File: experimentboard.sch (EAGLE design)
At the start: 173 parts, among them IC1 TL072P, IC2 LM317, IC3 LM337, IC4 TL072P, IC5 TL072P, IC6 TL072P, P1 PLR135/T9, U1 PCM1690, U2 DIR9001, U3 CAT24C256

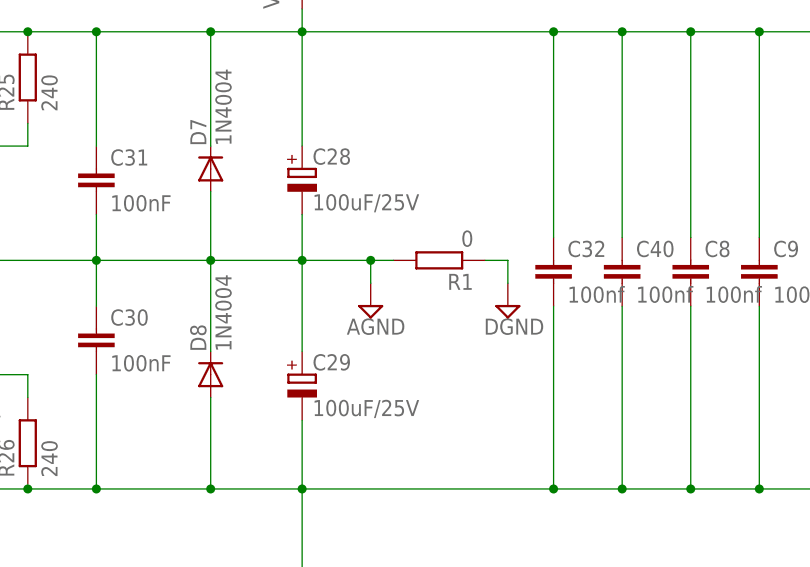
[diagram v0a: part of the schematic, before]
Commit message: Very nearly done
I added some power and ground planes and finished more routing.

Still a bit of decision making to do before I can finish it.
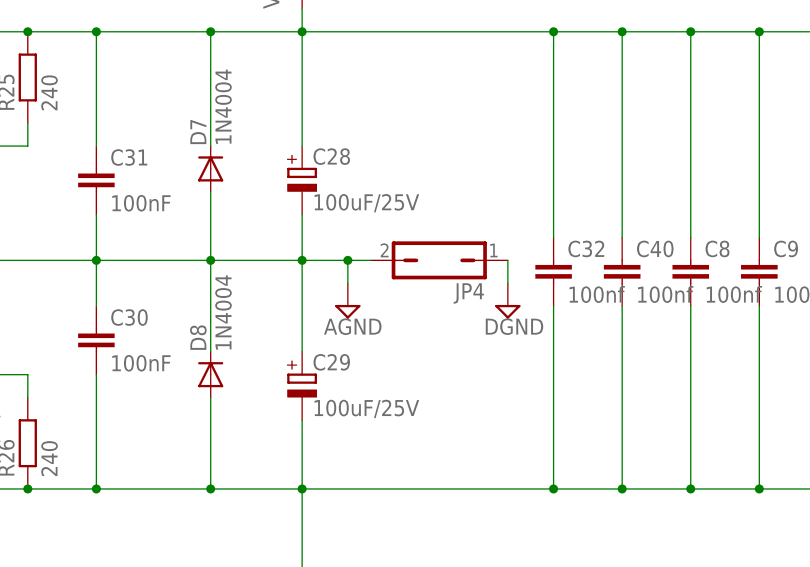
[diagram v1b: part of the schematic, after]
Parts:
- removed R1: 0, rcl:R-EU_0207/10
- added JP4: (no value), jumper:JP1Q
- P9: value BEAGLEBONEP9 -> P9
- renumbered U$2 to P9
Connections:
- net AGND: now also JP4.2; no longer R1.2
- net DGND: now also JP4.1; no longer R1.1
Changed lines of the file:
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@@
 <part name="R32" library="rcl" deviceset="R-EU_" device="0207/7" value="22"/>
 <part name="R3" library="rcl" deviceset="R-EU_" device="0207/7" value="10k"/>
-<part name="U$2" library="0000halfgaar" deviceset="BEAGLEBONEP9" device=""/>
+<part name="P9" library="0000halfgaar" deviceset="BEAGLEBONEP9" device="" value="P9"/>
 <part name="R35" library="rcl" deviceset="R-EU_" device="0207/7" value="22"/>
 <part name="R36" library="rcl" deviceset="R-EU_" device="0207/7" value="22"/>
@@
 <part name="SUPPLY14" library="supply2" deviceset="VDD" device=""/>
 <part name="SUPPLY31" library="supply2" deviceset="VDD" device=""/>
-<part name="R1" library="rcl" deviceset="R-EU_" device="0207/10" value="0"/>
 <part name="SUPPLY13" library="supply2" deviceset="DGND" device=""/>
 <part name="SUPPLY27" library="supply2" deviceset="VCC" device=""/>
@@
 <part name="C16" library="rcl" deviceset="CPOL-EU" device="E2-5" value="10 µF"/>
 <part name="C17" library="rcl" deviceset="CPOL-EU" device="E2-5" value="10 µF"/>
+<part name="JP4" library="jumper" deviceset="JP1Q" device=""/>
 </parts>
 <sheets>
@@
 </instance>
 <instance part="SUPPLY15" gate="G$1" x="-81.28" y="93.98" rot="R180"/>
-<instance part="SUPPLY16" gate="G$1" x="116.84" y="210.82"/>
+<instance part="SUPPLY16" gate="G$1" x="114.3" y="210.82"/>
 <instance part="AOUT" gate="-1" x="309.88" y="152.4" rot="R180"/>
 <instance part="AOUT" gate="-2" x="309.88" y="162.56" rot="R180"/>
@@
 <attribute name="VALUE" x="62.23" y="4.318" size="1.778" layer="96"/>
 </instance>
-<instance part="U$2" gate="G$1" x="-50.8" y="58.42"/>
+<instance part="P9" gate="G$1" x="-50.8" y="58.42"/>
 <instance part="R35" gate="G$1" x="63.5" y="93.98" smashed="yes">
 <attribute name="NAME" x="67.056" y="91.6686" size="1.778" layer="95"/>
@@
 <instance part="SUPPLY14" gate="G$1" x="22.86" y="43.18"/>
 <instance part="SUPPLY31" gate="G$1" x="30.48" y="43.18"/>
-<instance part="R1" gate="G$1" x="124.46" y="215.9" rot="R180"/>
 <instance part="SUPPLY13" gate="G$1" x="132.08" y="210.82"/>
 <instance part="SUPPLY27" gate="G$1" x="210.82" y="238.76" rot="R180"/>
@@
 <instance part="C16" gate="G$1" x="96.52" y="-187.96" rot="R90"/>
 <instance part="C17" gate="G$1" x="165.1" y="-83.82"/>
+<instance part="JP4" gate="A" x="124.46" y="215.9" rot="R90"/>
 </instances>
 <busses>
@@
 <pinref part="R32" gate="G$1" pin="1"/>
 <wire x1="68.58" y1="-119.38" x2="-15.24" y2="-119.38" width="0.1524" layer="91"/>
-<pinref part="U$2" gate="G$1" pin="DIN"/>
+<pinref part="P9" gate="G$1" pin="DIN"/>
 <wire x1="-30.48" y1="68.58" x2="-15.24" y2="68.58" width="0.1524" layer="91"/>
 <wire x1="-15.24" y1="68.58" x2="-15.24" y2="-119.38" width="0.1524" layer="91"/>
@@
 </segment>
 <segment>
-<pinref part="U$2" gate="G$1" pin="3.3V"/>
+<pinref part="P9" gate="G$1" pin="3.3V"/>
 <pinref part="SUPPLY19" gate="G$1" pin="VDD"/>
 <wire x1="-78.74" y1="86.36" x2="-91.44" y2="86.36" width="0.1524" layer="91"/>
@@
 </segment>
 <segment>
-<pinref part="U$2" gate="G$1" pin="DGND"/>
+<pinref part="P9" gate="G$1" pin="DGND"/>
 <pinref part="SUPPLY15" gate="G$1" pin="DGND"/>
 <wire x1="-78.74" y1="88.9" x2="-81.28" y2="88.9" width="0.1524" layer="91"/>
@@
 </segment>
 <segment>
-<pinref part="R1" gate="G$1" pin="1"/>
 <pinref part="SUPPLY13" gate="G$1" pin="DGND"/>
-<wire x1="129.54" y1="215.9" x2="132.08" y2="215.9" width="0.1524" layer="91"/>
 <wire x1="132.08" y1="215.9" x2="132.08" y2="213.36" width="0.1524" layer="91"/>
+<pinref part="JP4" gate="A" pin="1"/>
 </segment>
 <segment>
@@
 </segment>
 <segment>
-<wire x1="116.84" y1="215.9" x2="116.84" y2="213.36" width="0.1524" layer="91"/>
+<wire x1="114.3" y1="215.9" x2="114.3" y2="213.36" width="0.1524" layer="91"/>
 <wire x1="109.22" y1="205.74" x2="109.22" y2="215.9" width="0.1524" layer="91"/>
 <wire x1="109.22" y1="215.9" x2="109.22" y2="220.98" width="0.1524" layer="91"/>
-<wire x1="109.22" y1="215.9" x2="116.84" y2="215.9" width="0.1524" layer="91"/>
+<wire x1="109.22" y1="215.9" x2="114.3" y2="215.9" width="0.1524" layer="91"/>
 <wire x1="99.06" y1="205.74" x2="99.06" y2="215.9" width="0.1524" layer="91"/>
 <wire x1="99.06" y1="215.9" x2="99.06" y2="223.52" width="0.1524" layer="91"/>
@@
 <wire x1="55.88" y1="223.52" x2="55.88" y2="215.9" width="0.1524" layer="91"/>
 <pinref part="SUPPLY16" gate="G$1" pin="AGND"/>
-<pinref part="R1" gate="G$1" pin="2"/>
-<wire x1="119.38" y1="215.9" x2="116.84" y2="215.9" width="0.1524" layer="91"/>
-<junction x="116.84" y="215.9"/>
+<pinref part="JP4" gate="A" pin="2"/>
+<wire x1="116.84" y1="215.9" x2="114.3" y2="215.9" width="0.1524" layer="91"/>
+<junction x="114.3" y="215.9"/>
 </segment>
 <segment>
@@
 <wire x1="22.86" y1="17.78" x2="10.16" y2="17.78" width="0.1524" layer="91"/>
 <wire x1="10.16" y1="17.78" x2="10.16" y2="58.42" width="0.1524" layer="91"/>
-<pinref part="U$2" gate="G$1" pin="I2C_SCL"/>
+<pinref part="P9" gate="G$1" pin="I2C_SCL"/>
 <wire x1="10.16" y1="58.42" x2="-30.48" y2="58.42" width="0.1524" layer="91"/>
 <pinref part="R38" gate="G$1" pin="1"/>
@@
 <wire x1="30.48" y1="22.86" x2="76.2" y2="22.86" width="0.1524" layer="91"/>
 <wire x1="12.7" y1="22.86" x2="12.7" y2="55.88" width="0.1524" layer="91"/>
-<pinref part="U$2" gate="G$1" pin="I2C_SDA"/>
+<pinref part="P9" gate="G$1" pin="I2C_SDA"/>
 <wire x1="12.7" y1="55.88" x2="-30.48" y2="55.88" width="0.1524" layer="91"/>
 <pinref part="R39" gate="G$1" pin="1"/>
@@
 </segment>
 <segment>
-<pinref part="U$2" gate="G$1" pin="VDD_5V"/>
+<pinref part="P9" gate="G$1" pin="VDD_5V"/>
 <pinref part="SUPPLY28" gate="G$1" pin="VCC"/>
 <wire x1="-78.74" y1="83.82" x2="-101.6" y2="83.82" width="0.1524" layer="91"/>
@@
 <wire x1="17.78" y1="66.04" x2="-7.62" y2="66.04" width="0.1524" layer="91"/>
 <wire x1="-7.62" y1="66.04" x2="-7.62" y2="86.36" width="0.1524" layer="91"/>
-<pinref part="U$2" gate="G$1" pin="AHCLKX"/>
+<pinref part="P9" gate="G$1" pin="AHCLKX"/>
 <wire x1="-7.62" y1="86.36" x2="-30.48" y2="86.36" width="0.1524" layer="91"/>
 </segment>
@@
 <wire x1="68.58" y1="-109.22" x2="-12.7" y2="-109.22" width="0.1524" layer="91"/>
 <wire x1="-12.7" y1="-109.22" x2="-12.7" y2="71.12" width="0.1524" layer="91"/>
-<pinref part="U$2" gate="G$1" pin="FSR"/>
+<pinref part="P9" gate="G$1" pin="FSR"/>
 <wire x1="-12.7" y1="71.12" x2="-30.48" y2="71.12" width="0.1524" layer="91"/>
 </segment>
@@
 <segment>
 <pinref part="U1" gate="U$1" pin="RST"/>
-<pinref part="U$2" gate="G$1" pin="RESET(GPIO1_16)"/>
+<pinref part="P9" gate="G$1" pin="RESET(GPIO1_16)"/>
 <wire x1="-30.48" y1="50.8" x2="-2.54" y2="50.8" width="0.1524" layer="91"/>
 <wire x1="-2.54" y1="50.8" x2="-2.54" y2="48.26" width="0.1524" layer="91"/>
@@
 <pinref part="R31" gate="G$1" pin="1"/>
 <wire x1="68.58" y1="-114.3" x2="-10.16" y2="-114.3" width="0.1524" layer="91"/>
-<pinref part="U$2" gate="G$1" pin="ACLKR"/>
+<pinref part="P9" gate="G$1" pin="ACLKR"/>
 <wire x1="-30.48" y1="73.66" x2="-10.16" y2="73.66" width="0.1524" layer="91"/>
 <wire x1="-10.16" y1="73.66" x2="-10.16" y2="-114.3" width="0.1524" layer="91"/>
@@
 <net name="DOUT" class="0">
 <segment>
-<pinref part="U$2" gate="G$1" pin="DOUT"/>
+<pinref part="P9" gate="G$1" pin="DOUT"/>
 <wire x1="-30.48" y1="78.74" x2="7.62" y2="78.74" width="0.1524" layer="91"/>
 <wire x1="7.62" y1="78.74" x2="7.62" y2="83.82" width="0.1524" layer="91"/>
@@
 <net name="AHCLKX" class="0">
 <segment>
-<pinref part="U$2" gate="G$1" pin="FSX"/>
+<pinref part="P9" gate="G$1" pin="FSX"/>
 <wire x1="-30.48" y1="81.28" x2="-2.54" y2="81.28" width="0.1524" layer="91"/>
 <wire x1="-2.54" y1="81.28" x2="-2.54" y2="93.98" width="0.1524" layer="91"/>
@@
 <segment>
 <wire x1="2.54" y1="88.9" x2="2.54" y2="83.82" width="0.1524" layer="91"/>
-<pinref part="U$2" gate="G$1" pin="ACLKX"/>
+<pinref part="P9" gate="G$1" pin="ACLKX"/>
 <wire x1="2.54" y1="83.82" x2="-30.48" y2="83.82" width="0.1524" layer="91"/>
 <pinref part="R36" gate="G$1" pin="1"/>
@@
 <wire x1="83.82" y1="-63.5" x2="-17.78" y2="-63.5" width="0.1524" layer="91"/>
 <wire x1="-17.78" y1="-63.5" x2="-17.78" y2="66.04" width="0.1524" layer="91"/>
-<pinref part="U$2" gate="G$1" pin="DIR_AUDIO(GPIO1_19)"/>
+<pinref part="P9" gate="G$1" pin="DIR_AUDIO(GPIO1_19)"/>
 <wire x1="-17.78" y1="66.04" x2="-30.48" y2="66.04" width="0.1524" layer="91"/>
 </segment>
@@
 <net name="CAPE_I2C_SDA" class="0">
 <segment>
-<pinref part="U$2" gate="G$1" pin="EEPROM_I2C_SDA"/>
+<pinref part="P9" gate="G$1" pin="EEPROM_I2C_SDA"/>
 <wire x1="-30.48" y1="40.64" x2="-27.94" y2="40.64" width="0.1524" layer="91"/>
 <wire x1="-27.94" y1="40.64" x2="-27.94" y2="0" width="0.1524" layer="91"/>
@@
 <wire x1="-38.1" y1="2.54" x2="-25.4" y2="2.54" width="0.1524" layer="91"/>
 <wire x1="-25.4" y1="2.54" x2="-25.4" y2="43.18" width="0.1524" layer="91"/>
-<pinref part="U$2" gate="G$1" pin="EEPROM_I2C_SCL"/>
+<pinref part="P9" gate="G$1" pin="EEPROM_I2C_SCL"/>
 <wire x1="-25.4" y1="43.18" x2="-30.48" y2="43.18" width="0.1524" layer="91"/>
 <pinref part="R8" gate="G$1" pin="1"/>

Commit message: Fixed 5mm caps, fixed DRC errors
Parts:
- 1_C1, 1_C2, 2_C1, 2_C2, 3_C1, 3_C2, 4_C1, 4_C2, 5_C1, 5_C2, 6_C1, 6_C2, 7_C1, 7_C2, 8_C1, 8_C2: device rcl:CPOL-EUE1.8-4 -> rcl:CPOL-EUE2-5
